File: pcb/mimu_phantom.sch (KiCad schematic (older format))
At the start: 0 parts

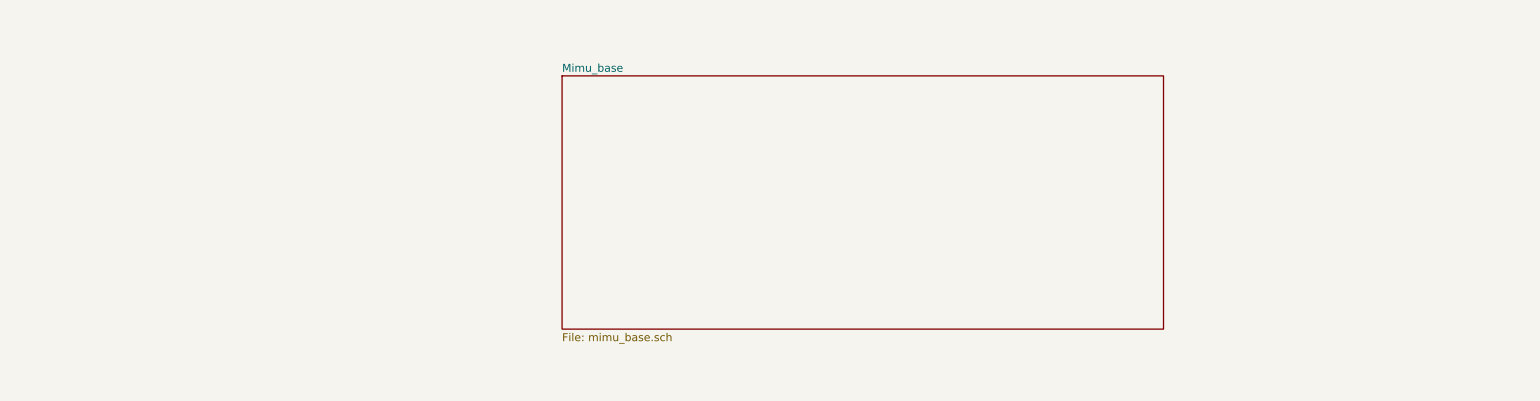
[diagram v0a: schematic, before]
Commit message: I hope this did not break everything
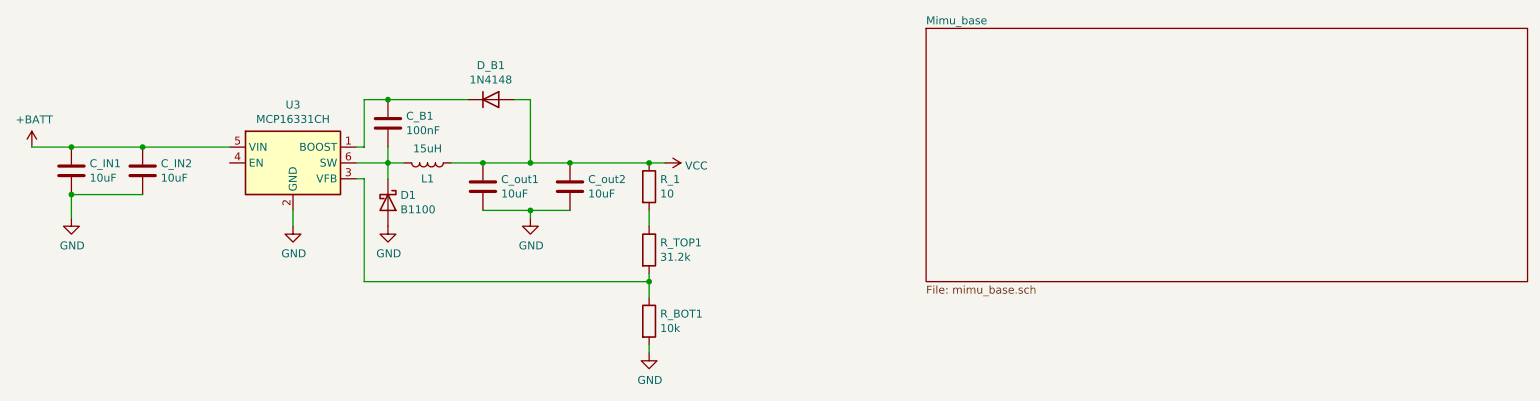
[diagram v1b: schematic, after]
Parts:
- added C_B1: 100nF, Capacitor_SMD:C_1206_3216Metric_Pad1.42x1.75mm_HandSolder, symbol Device:C
- added C_IN1, C_IN2, C_out1, C_out2: 10uF, Capacitor_SMD:C_1206_3216Metric_Pad1.42x1.75mm_HandSolder, symbol Device:C
- added D1: B1100, Diode_SMD:D_SMA, symbol Device:D_Schottky
- added D_B1: 1N4148, Diode_SMD:D_SMA, symbol Device:D
- added L1: 15uH, Inductor_SMD:L_7.3x7.3_H4.5, symbol Device:L
- added R_1: 10, Resistor_SMD:R_1206_3216Metric_Pad1.42x1.75mm_HandSolder, symbol Device:R
- added R_BOT1: 10k, Resistor_SMD:R_1206_3216Metric_Pad1.42x1.75mm_HandSolder, symbol Device:R
- added R_TOP1: 31.2k, Resistor_SMD:R_1206_3216Metric_Pad1.42x1.75mm_HandSolder, symbol Device:R
- added U3: MCP16331CH, Package_TO_SOT_SMD:SOT-23-6, symbol Regulator_Switching:MCP16331CH
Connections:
- new net: C_B1.1, D_B1.1 (K), U3.1 (BOOST)
- new net: R_BOT1.1, R_TOP1.2, U3.3 (VFB)
- new net: C_B1.2, D1.1 (K), L1.2, U3.6 (SW)
- new net: R_1.2, R_TOP1.1
- new net +BATT: C_IN1.1, C_IN2.1, U3.5 (VIN)
- new net GND: C_IN1.2, C_IN2.2, C_out1.2, C_out2.2, D1.2 (A), R_BOT1.2, U3.2 (GND)
- new net VCC: C_out1.1, C_out2.1, D_B1.2 (A), L1.1, R_1.1
